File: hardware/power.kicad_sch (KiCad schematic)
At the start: 48 parts, among them J8 USB_C_Receptacle_USB2.0_16P, Q1 AO3400A, U10 EL817S1C, U12 USBLC6-2SC6, U2 IP5306, U7 AOZ1280CI

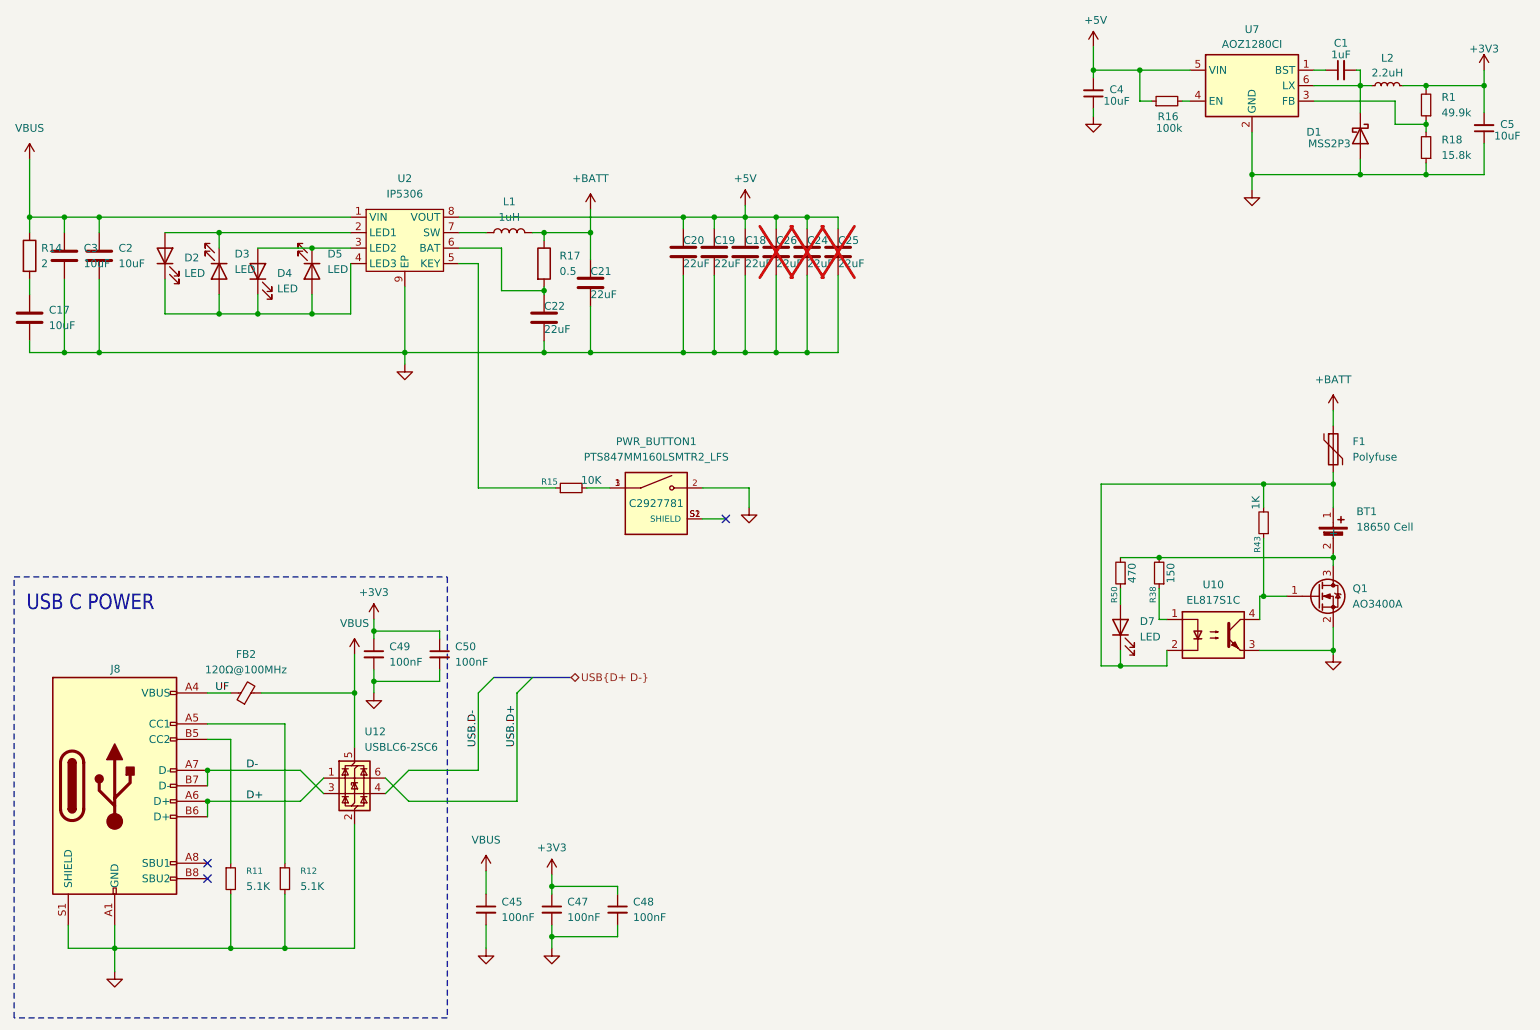
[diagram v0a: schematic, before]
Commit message: Passing DRC
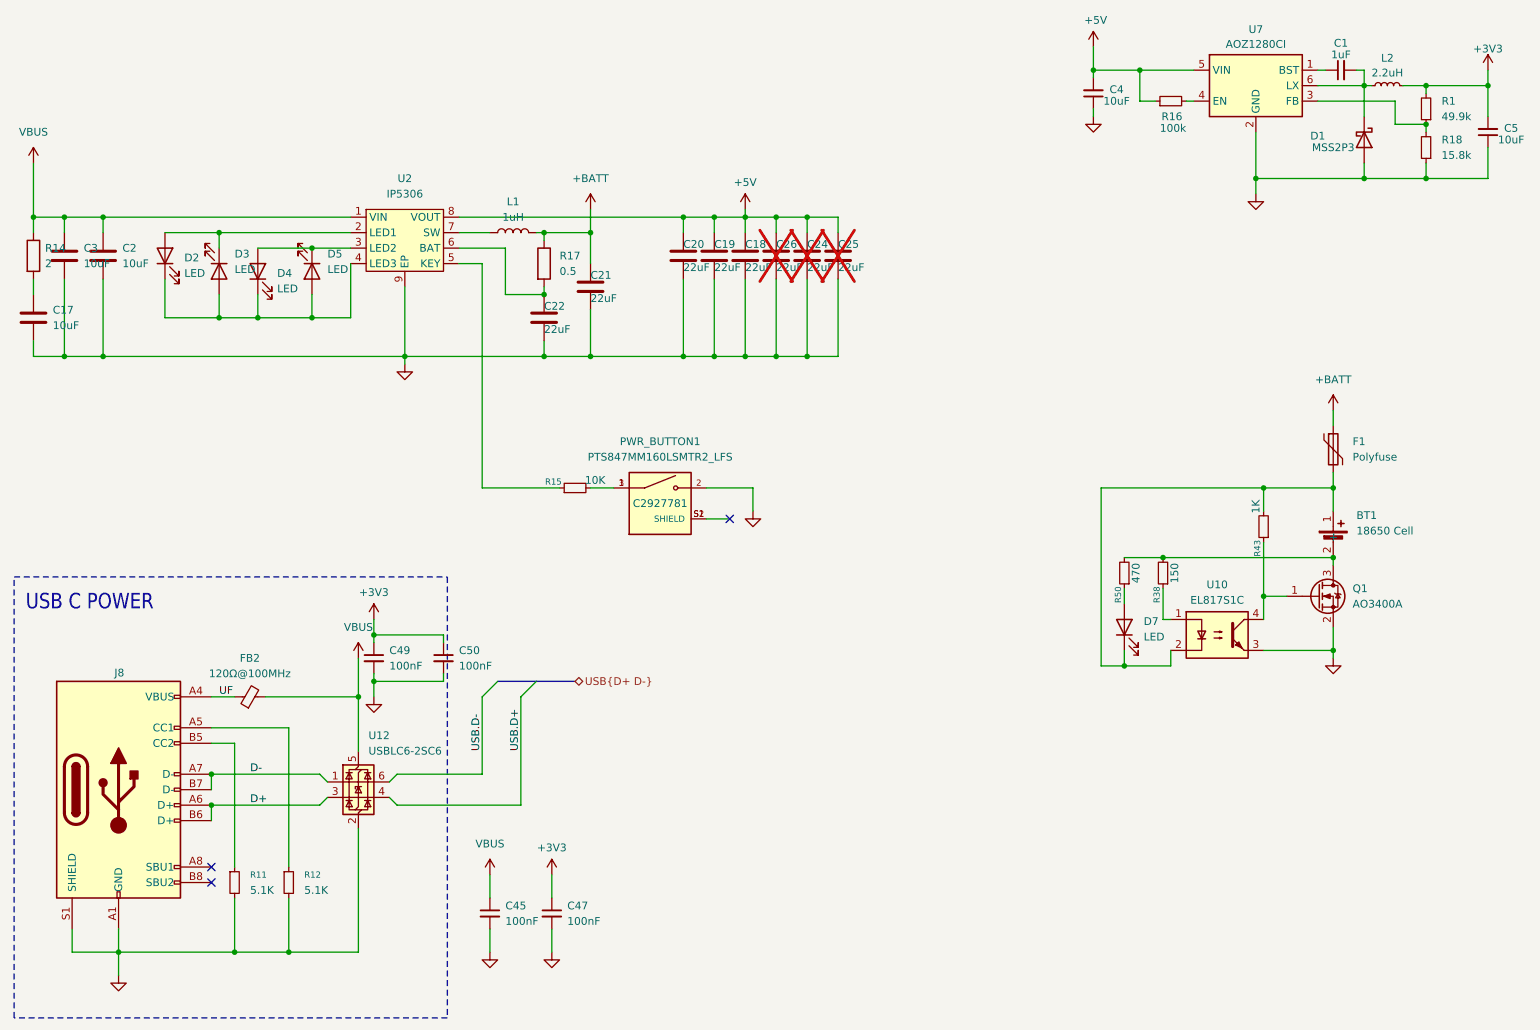
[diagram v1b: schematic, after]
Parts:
- removed C48: 100nF, Capacitor_SMD:C_0402_1005Metric, symbol Device:C_Small
- R16: footprint (none) -> Resistor_SMD:R_0402_1005Metric
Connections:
- net D+: now also U12.3 (I/O2); no longer U12.1 (I/O1)
- net D-: now also U12.1 (I/O1); no longer U12.3 (I/O2)
- net USB.D+: now also U12.4 (I/O2); no longer U12.6 (I/O1)
- net USB.D-: now also U12.6 (I/O1); no longer U12.4 (I/O2)
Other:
- moved on the sheet: BT1, C17, C18, C19, C2, C20, C21, C24, C25, C26, C45, C47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
